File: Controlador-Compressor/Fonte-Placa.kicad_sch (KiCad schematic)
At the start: 13 parts, among them U2 LM2596S-5, U7 AMS1117-3.3

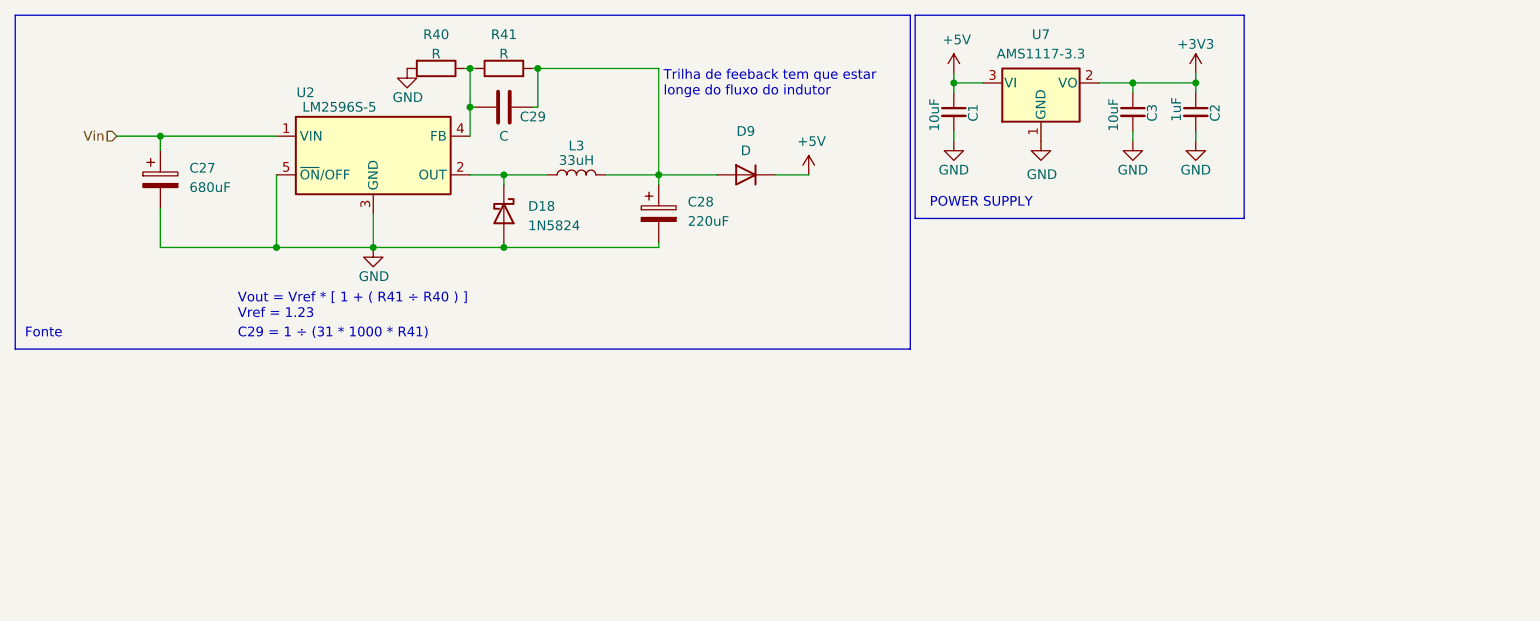
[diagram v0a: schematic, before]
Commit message: terminei escopo do projeto
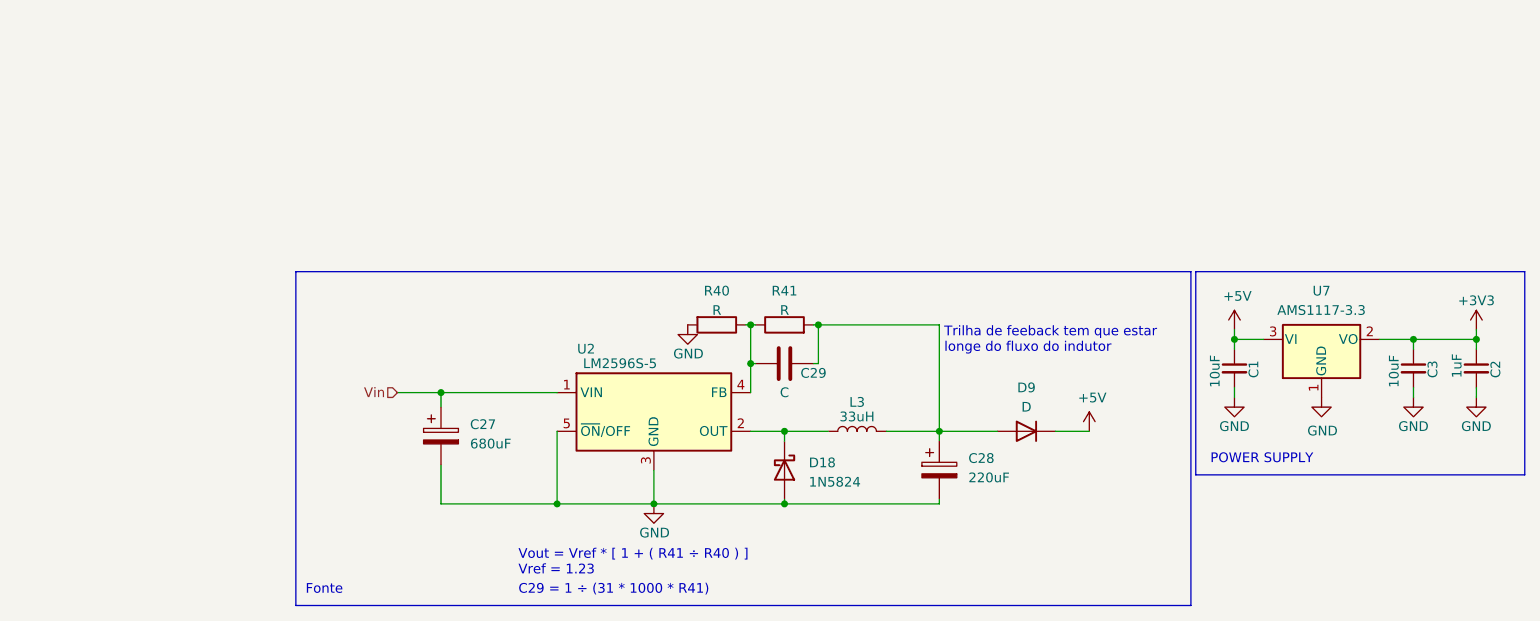
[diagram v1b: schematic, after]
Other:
- company: (none) -> Linear Compressores
- title: (none) -> Controlador Compressor
- moved on the sheet: C1, C2, C27, C28, C29, C3, D18, D9, L3, R40, R41, U2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
